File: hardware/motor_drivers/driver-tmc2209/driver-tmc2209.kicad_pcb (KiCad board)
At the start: 4 copper layers, 30 x 24 mm, 33 parts, among them M1 JST XH, T10 CS0, T11 STEP, T12 GND, T13 DIR, T14 EN, T17 DIAG, T5 GND, T8 VCC, T9 Therm, U1 TMC2209-LA

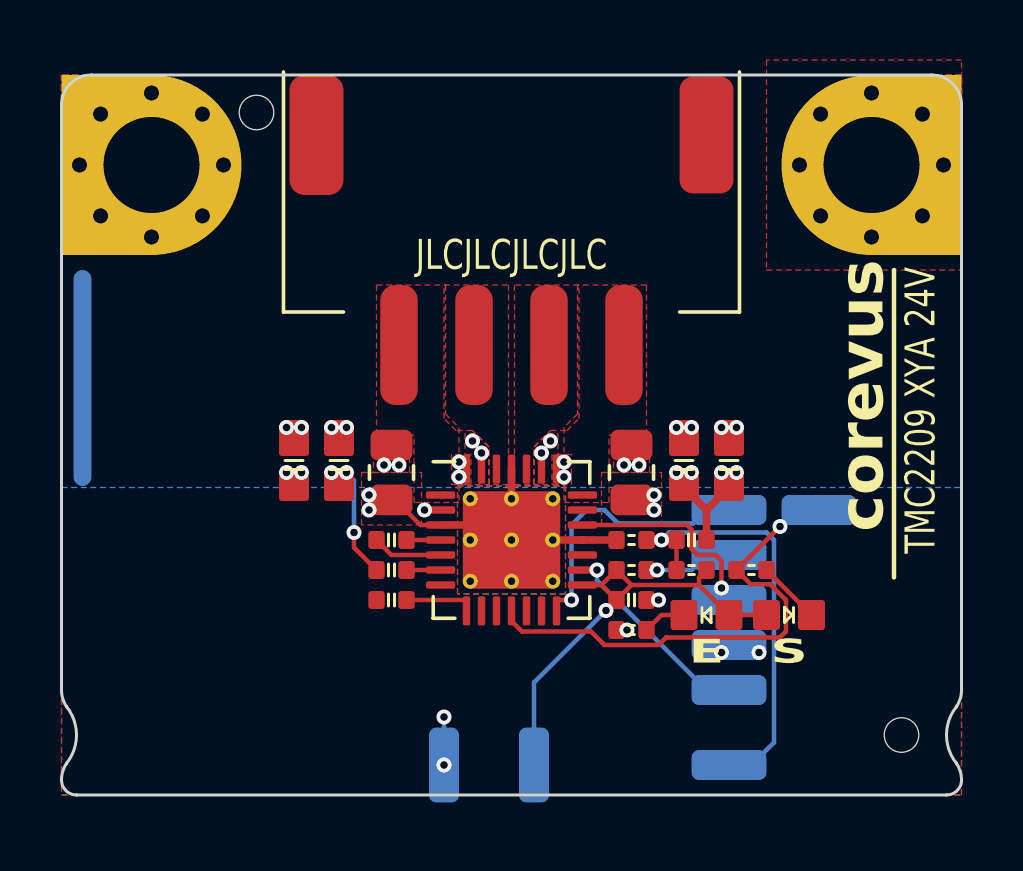
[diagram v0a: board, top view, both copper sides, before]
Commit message: should be up to date for cvg v0.6 and latest protected drivers
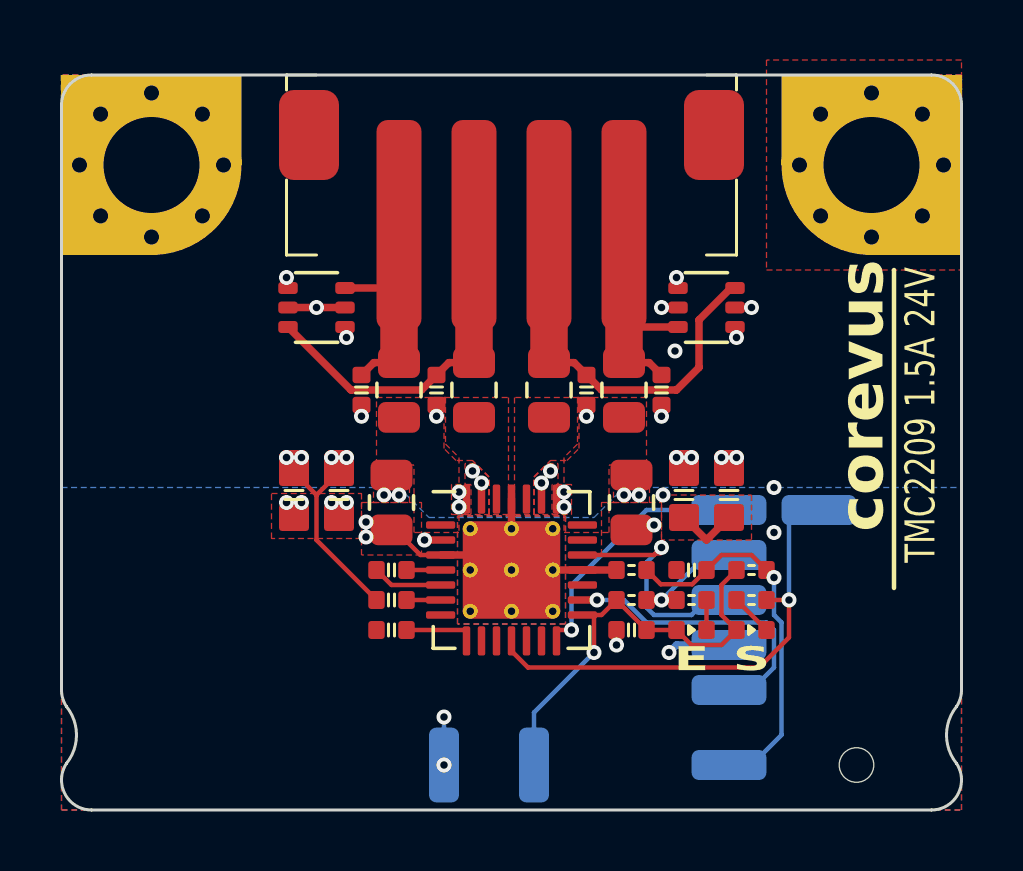
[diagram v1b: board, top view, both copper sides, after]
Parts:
- removed H4: MountingHole, corevus:ToolingHole
- removed M1: JST XH, corevus:XKB_X8821WRS-04
- added C10: 1nF 100V, PCM_ME_passives:0402C, F.Cu at (137.5, 67.5)
- added C11: 1nF 100V, PCM_ME_passives:0402C, F.Cu at (132.5, 67.5)
- added C12: 1nF 100V, PCM_ME_passives:0402C, F.Cu at (130.0, 67.5)
- added C9: 1nF 100V, PCM_ME_passives:0402C, F.Cu at (140.0, 67.5)
- added D3: BAV99S, Package_TO_SOT_SMD:SOT-363_SC-70-6, F.Cu at (141.5, 64.8)
- added D4: BAV99S, Package_TO_SOT_SMD:SOT-363_SC-70-6, F.Cu at (128.5, 64.8)
- added FB1: 30Ω@100MHz, Resistor_SMD:R_0805_2012Metric, F.Cu at (138.8, 67.5)
- added FB2: 30Ω@100MHz, Resistor_SMD:R_0805_2012Metric, F.Cu at (136.2, 67.5)
- added FB3: 30Ω@100MHz, Resistor_SMD:R_0805_2012Metric, F.Cu at (133.8, 67.5)
- added FB4: 30Ω@100MHz, Resistor_SMD:R_0805_2012Metric, F.Cu at (131.2, 67.5)
- added J1: XH, corevus:XH_1x04_SMD_Vertical, F.Cu at (135.0, 61.0)
- D1: value G -> Red; footprint AlphaLib:0603LED -> AlphaLib:0402LED
- D2: value Y -> Green; footprint AlphaLib:0603LED -> AlphaLib:0402LED
- H1, H2: footprint corevus:MountingHole_M3_Driver -> corevus:MountingHole_M3_Driver_Corner
- H3: value MountingHole -> Tooling Hole
- moved R1 2.24 mm to (141.0, 74.5)
- moved R20 2.00 mm to (143.0, 73.5), turned to 180 degrees
- moved H3 1.80 mm to (146.5, 80.0)
- moved D2 1.35 mm to (143.0, 75.5)
- moved C13 1.00 mm to (141.0, 73.5), turned to 180 degrees
- moved C1 1.00 mm to (139.0, 75.5), turned to 180 degrees
- moved C2 1.00 mm to (131.0, 75.5)
- moved C3 1.00 mm to (131.0, 74.5)
- moved C4 1.00 mm to (131.0, 73.5)
- moved C5 1.00 mm to (142.2, 71.0)
- moved C6 1.00 mm to (140.8, 71.0)
- moved C7 1.00 mm to (129.2, 71.0)
- moved C8 1.00 mm to (127.8, 71.0)
- moved R16 1.00 mm to (143.0, 74.5), turned to 0 degrees
- moved R2 1.00 mm to (139.0, 74.5)
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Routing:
- net /A1': track 0.00 -> 13.2 mm
- net /B1': track 0.00 -> 11.7 mm
- net /B2': track 0.00 -> 7.51 mm
- net /A2': track 0.00 -> 7.51 mm
- net +24V: track 7.31 -> 13.4 mm, vias 13 -> 15
- net /THERM: track 14.8 -> 11.6 mm
- net /Step: track 6.75 -> 9.86 mm
- net GND: track 17.0 -> 14.6 mm, vias 17 -> 22
- net /~{En}: track 13.3 -> 12.0 mm, vias 3 -> 2
- net VCC: track 15.6 -> 14.4 mm
- net Net-(D2-K): track 2.12 -> 1.41 mm
- net /UART: track 8.09 -> 8.65 mm
- net (no net): vias 0 -> 1
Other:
- board size 30 x 24 mm -> 30 x 24.5 mm
- board text added: "3V3"
- board text added: "A"
- board text added: "DIR"
- board text added: "EN"
- board text added: "GND"
- board text added: "NOT FOR PRODUCTION USE MERIDI ENGINEERING MAY 2024 TMC2209 2ϕ STEPPER DRIVER 1.5A 24V MAX CV·24·08·19"
- board text added: "STALL"
- board text added: "STEP"
- board text added: "THERM"
- board text added: "TMC2209 1.5A 24V"
- board text added: "UART"
- board text removed: "CV·24·08·19·AA"
- board text removed: "JLCJLCJLCJLC"
- board text removed: "NOT FOR PRODUCTION USE"
- board text removed: "TMC2209 XYA 24V"
